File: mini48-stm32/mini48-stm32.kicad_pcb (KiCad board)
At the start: 2 copper layers, 78.9 x 19.8 mm, 37 parts, among them J1 MINI-USB, J2 Conn_01x20, J3 Conn_01x20, J4 Conn_02x03_Odd_Even, P201 CONN_4, P202 JUMPER, U1 STM32F103C8, U2 NUF2101MT1G, U201 SN65HVD230, U3 LM2937, X1 8MHz, X2 32.768KHz

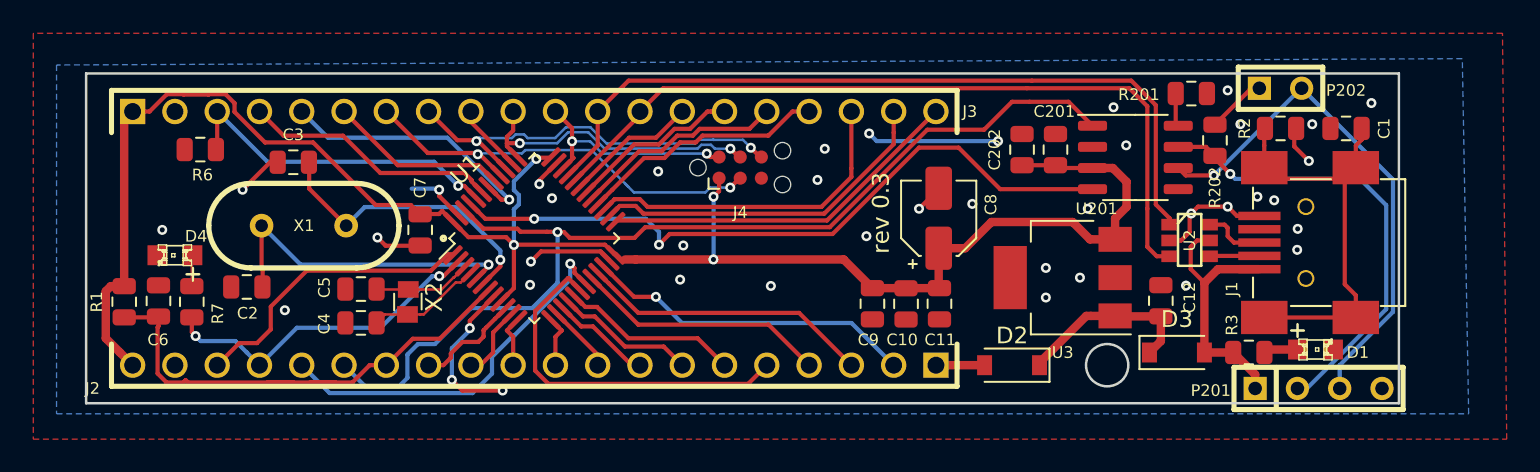
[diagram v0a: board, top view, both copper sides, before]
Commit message: progress
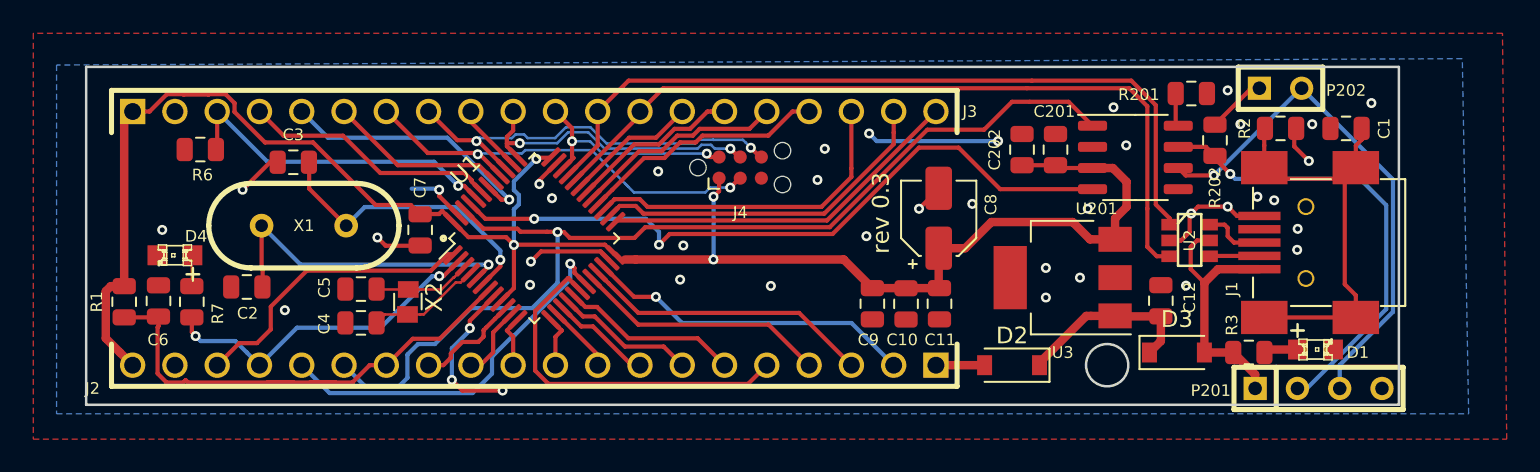
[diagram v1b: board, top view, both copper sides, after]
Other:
- board size 78.9 x 19.8 mm -> 78.9 x 20.3 mm
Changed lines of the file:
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@@
   )
   (setup
-    (last_trace_width 0.254)
+    (last_trace_width 0.1524)
     (user_trace_width 0.254)
     (user_trace_width 0.508)
@@
     (effects (font (size 1.016 1.016) (thickness 0.2032)) (justify left mirror))
   )
-  (gr_line (start 109.474 98.806) (end 109.474 78.994) (angle 90) (layer Edge.Cuts) (width 0.15))
-  (gr_line (start 188.341 98.806) (end 109.474 98.806) (angle 90) (layer Edge.Cuts) (width 0.15))
-  (gr_line (start 188.341 78.994) (end 188.341 98.806) (angle 90) (layer Edge.Cuts) (width 0.15))
-  (gr_line (start 109.474 78.994) (end 188.341 78.994) (angle 90) (layer Edge.Cuts) (width 0.15))
+  (gr_line (start 109.474 98.9) (end 109.474 78.6) (angle 90) (layer Edge.Cuts) (width 0.15))
+  (gr_line (start 188.341 98.9) (end 109.474 98.9) (angle 90) (layer Edge.Cuts) (width 0.15))
+  (gr_line (start 188.341 78.6) (end 188.341 98.9) (angle 90) (layer Edge.Cuts) (width 0.15))
+  (gr_line (start 109.474 78.6) (end 188.341 78.6) (angle 90) (layer Edge.Cuts) (width 0.15))
   (via (at 131.8274 85.7486) (size 0.6) (drill 0.3) (layers F.Cu B.Cu) (net 1))
   (segment (start 131.8274 85.7487) (end 131.8274 85.7486) (width 0.254) (layer F.Cu) (net 1))
